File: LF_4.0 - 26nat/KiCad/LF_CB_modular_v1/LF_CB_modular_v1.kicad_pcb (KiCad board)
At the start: 2 copper layers, 24 parts, among them J1 Conn_QTR16, J10 Conn_01x02, J11 Conn_01x10, J2 Conn_Arducam_MEGA_3mpx, J3 Conn_TB6612FNG_IC, J4 Conn_01x02, J8 Conn_01x01, J9 Conn_01x01, M1 Motor_DC, M2 Motor_DC, Q1 IRF4905, SW1 SW_SPDT, U1 Teensy4.1, U2 LM7805_TO220

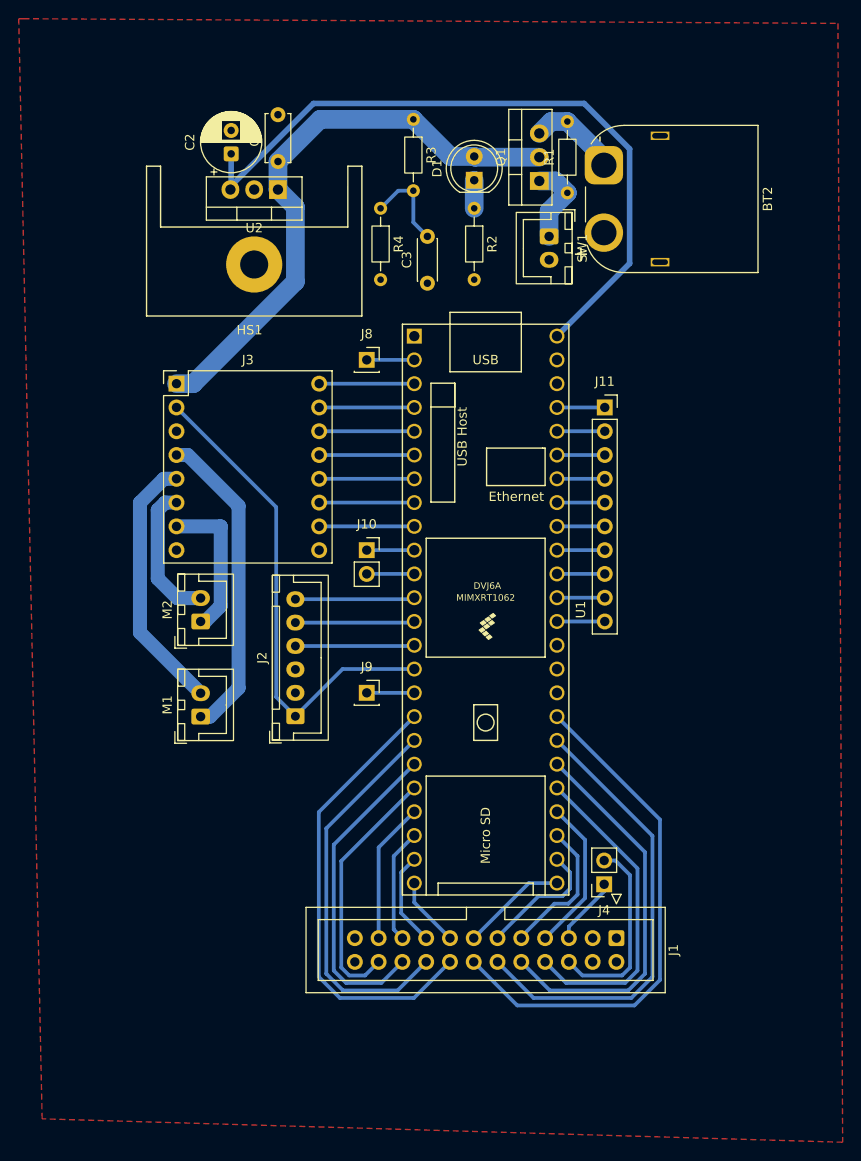
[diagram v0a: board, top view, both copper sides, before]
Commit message: power modul finishing
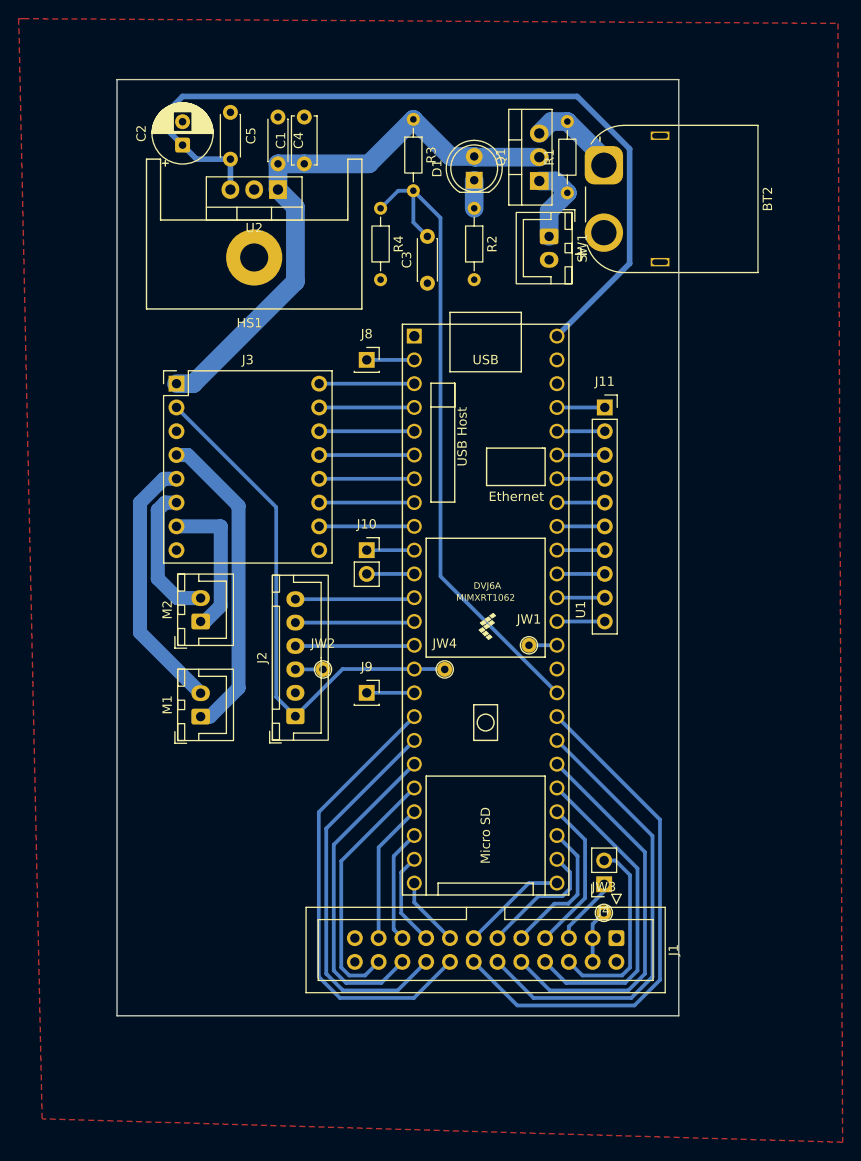
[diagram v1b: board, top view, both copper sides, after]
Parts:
- added C4: C_100n, Capacitor_THT:C_Disc_D4.3mm_W1.9mm_P5.00mm, F.Cu at (56.2, 45.0)
- added C5: C_100n, Capacitor_THT:C_Disc_D4.3mm_W1.9mm_P5.00mm, F.Cu at (51.1, 44.5)
- added JW1: Cam_SCK, Linefollower:Jumper_pin, F.Cu at (83.0, 101.4)
- added JW2: Cam_SCK, Linefollower:Jumper_pin, F.Cu at (61.0, 104.0)
- added JW3: 3V3, Linefollower:Jumper_pin, F.Cu at (91.0, 130.0)
- added JW4: 3V3, Linefollower:Jumper_pin, F.Cu at (74.0, 104.0)
- U2: value LM7805_TO220 -> LM2940CT-5.0 _TO220
- moved C2 5.27 mm to (46.0, 48.0)
- moved C1 2.82 mm to (59.0, 50.0)
- moved HS1 0.75 mm to (53.6, 60.0)
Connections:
- BT2 pad : (no net) -> /GND
- J1 pad 3: /3V3 -> Net-(JW3-Pin_1)
- J1 pad 4: /3V3 -> Net-(JW3-Pin_1)
- J2 pad 3: /Cam_SCK -> Net-(J2-SCK)
- U1 pad 35: /Cam_SCK -> Net-(JW1-Pin_1)
- U1 pad 46: /3V3 -> unconnected-(U1-3V3-Pad46)
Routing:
- net /BATT_SENSE: track 9.78 -> 69.8 mm
- net /5V: track 75.7 -> 88.8 mm
- net Net-(JW3-Pin_1): track 0.00 -> 5.74 mm
- net /3V3: track 53.0 -> 56.3 mm
- net Net-(JW1-Pin_1): track 0.00 -> 2.99 mm
- net Net-(J2-SCK): track 0.00 -> 2.95 mm
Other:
- board outline added: 60 x 100 mm
